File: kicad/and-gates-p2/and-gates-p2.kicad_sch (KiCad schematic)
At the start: 28 parts

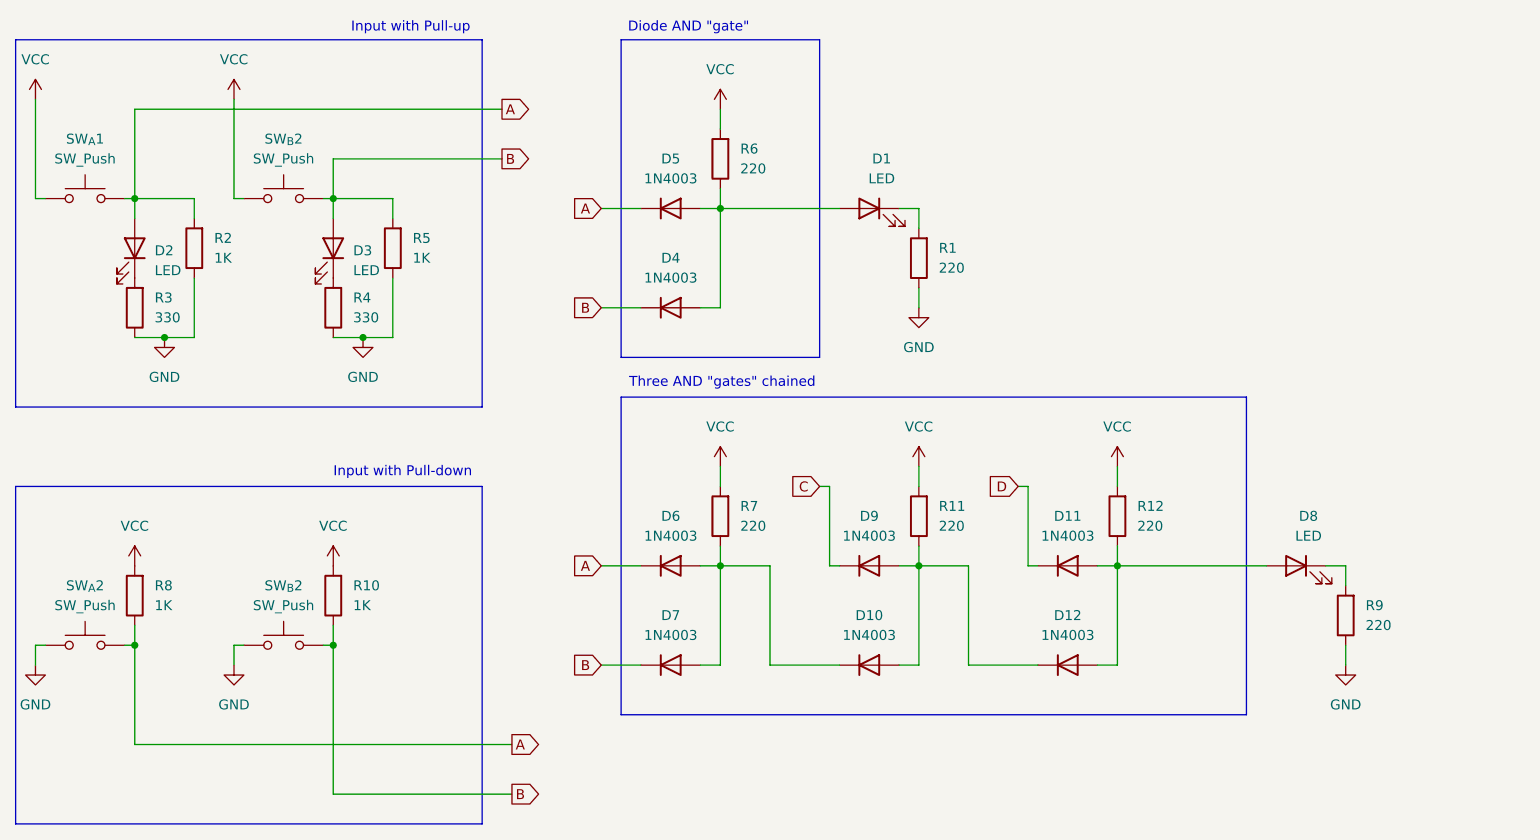
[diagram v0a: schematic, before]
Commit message: Update and export schematics
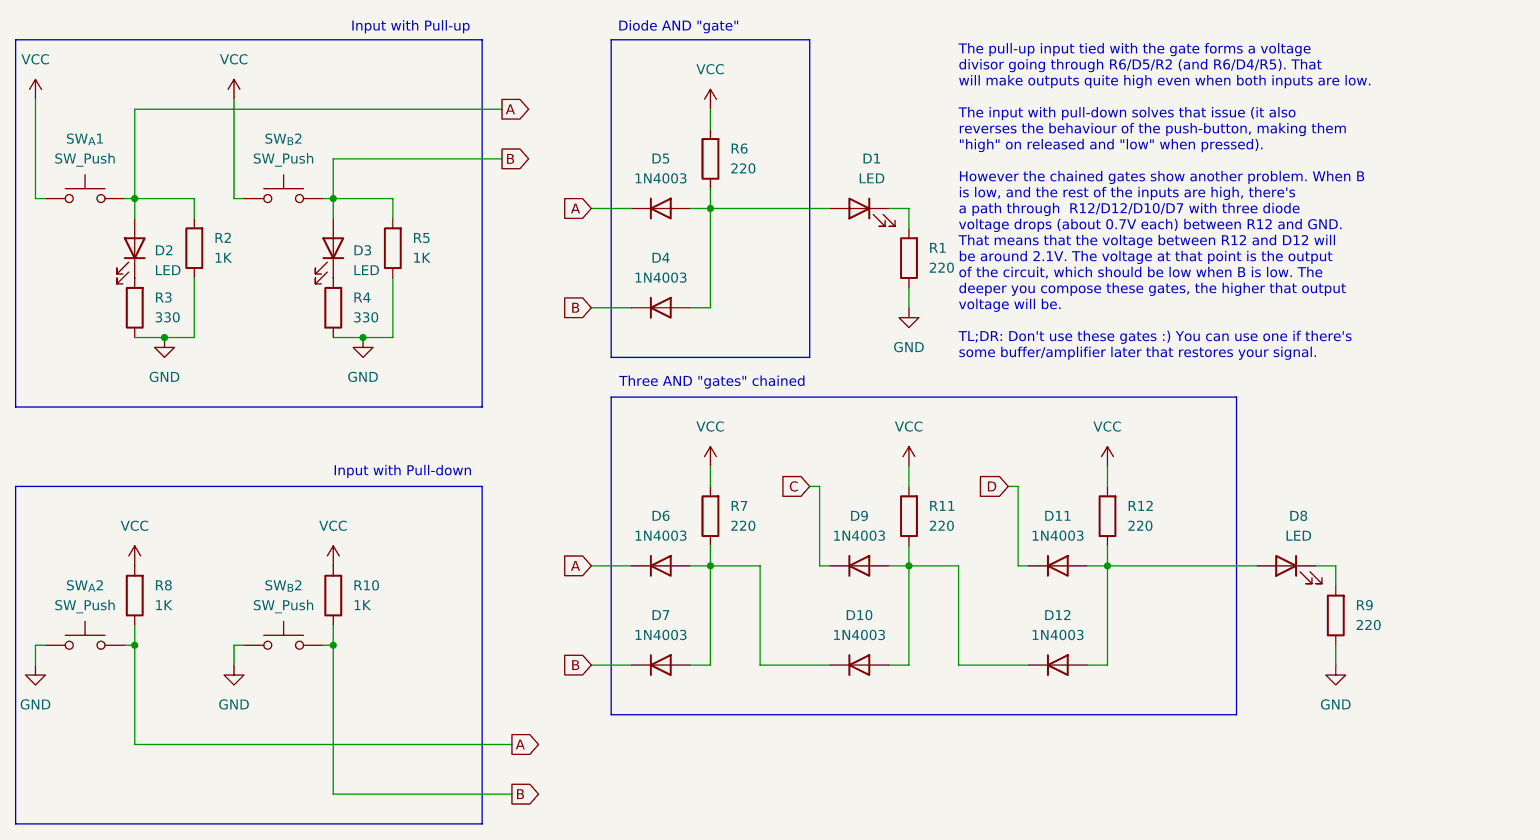
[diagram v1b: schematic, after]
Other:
- note added: "The pull-up input tied with the gate forms a voltage divisor going through R6/D5/R2 (and R6/D4/R5). That will make outputs quite high even when both inputs are low. The input with pull-down solves that issue (it also reverses the behaviour of the push-button, making them "high" on released and "low" when pressed). However the chained gates show another problem. When B is low, and the rest of the 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"
- company: (none) -> Silicon Chronicles
- title: Diodes & Diodes (Building AND gates the wrong way: Part 2) -> Diodes & Diodes
- moved on the sheet: D1, D10, D11, D12, D4, D5, D6, D7, D8, D9, R1, R11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
